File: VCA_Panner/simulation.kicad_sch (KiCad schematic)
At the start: 38 parts, among them U4 TL074, U5 TL074

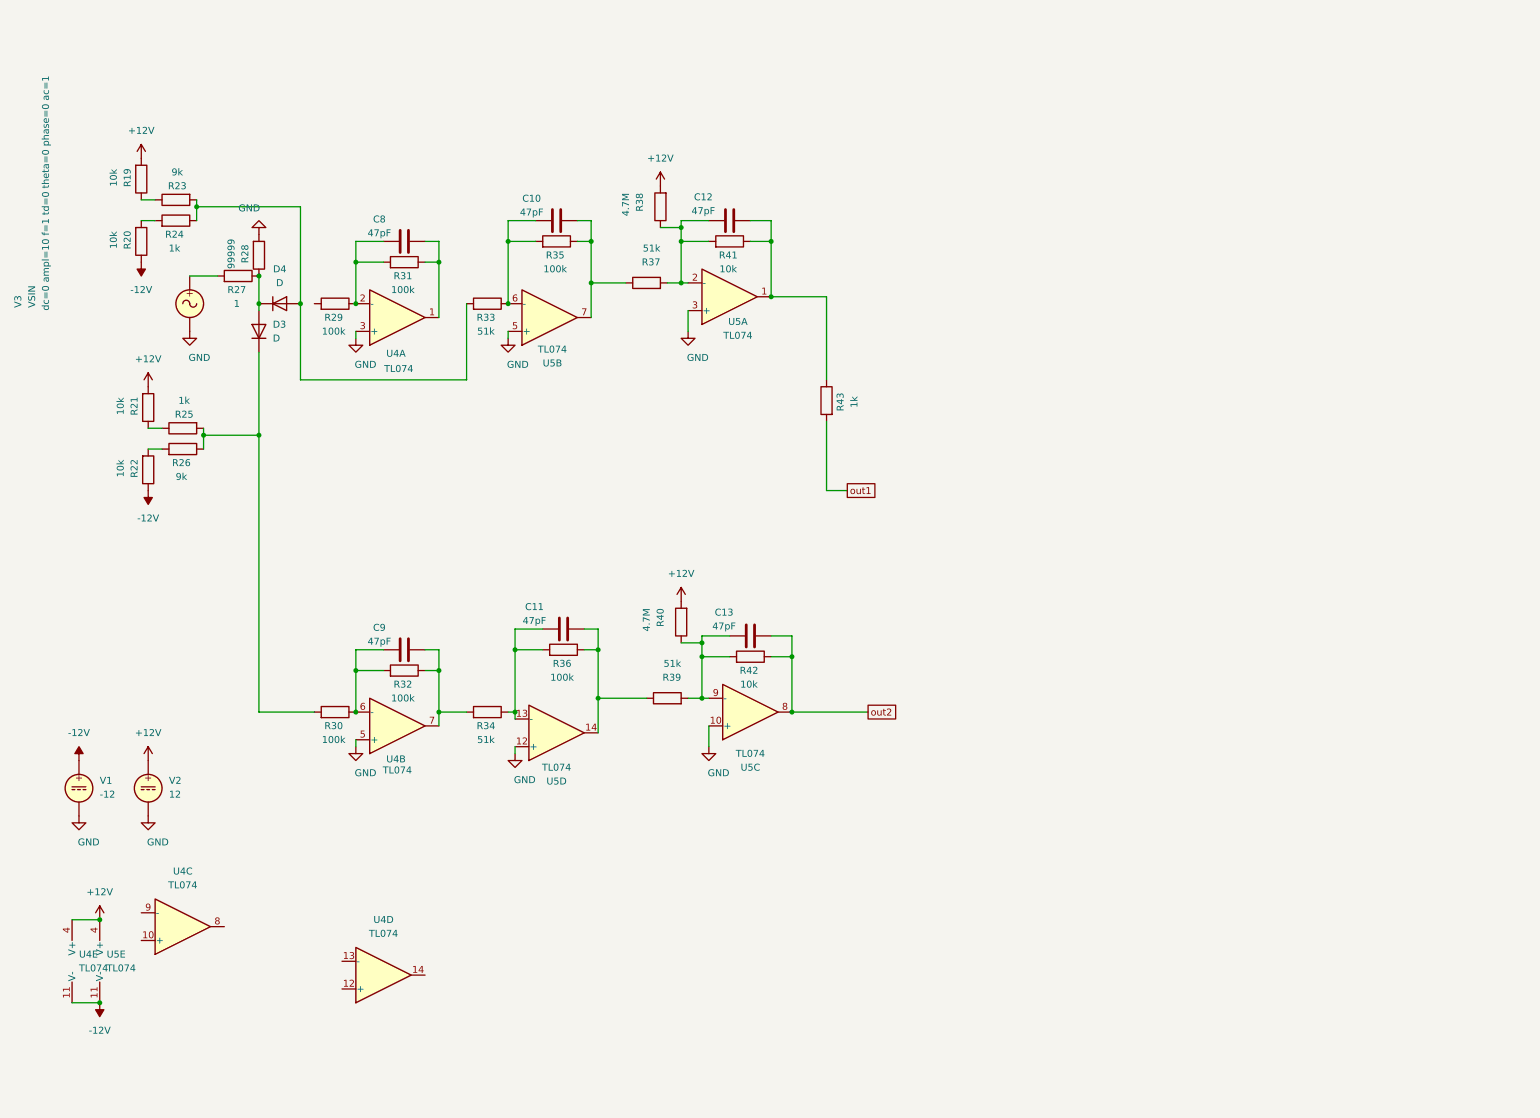
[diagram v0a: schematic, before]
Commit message: feitw bugfixes
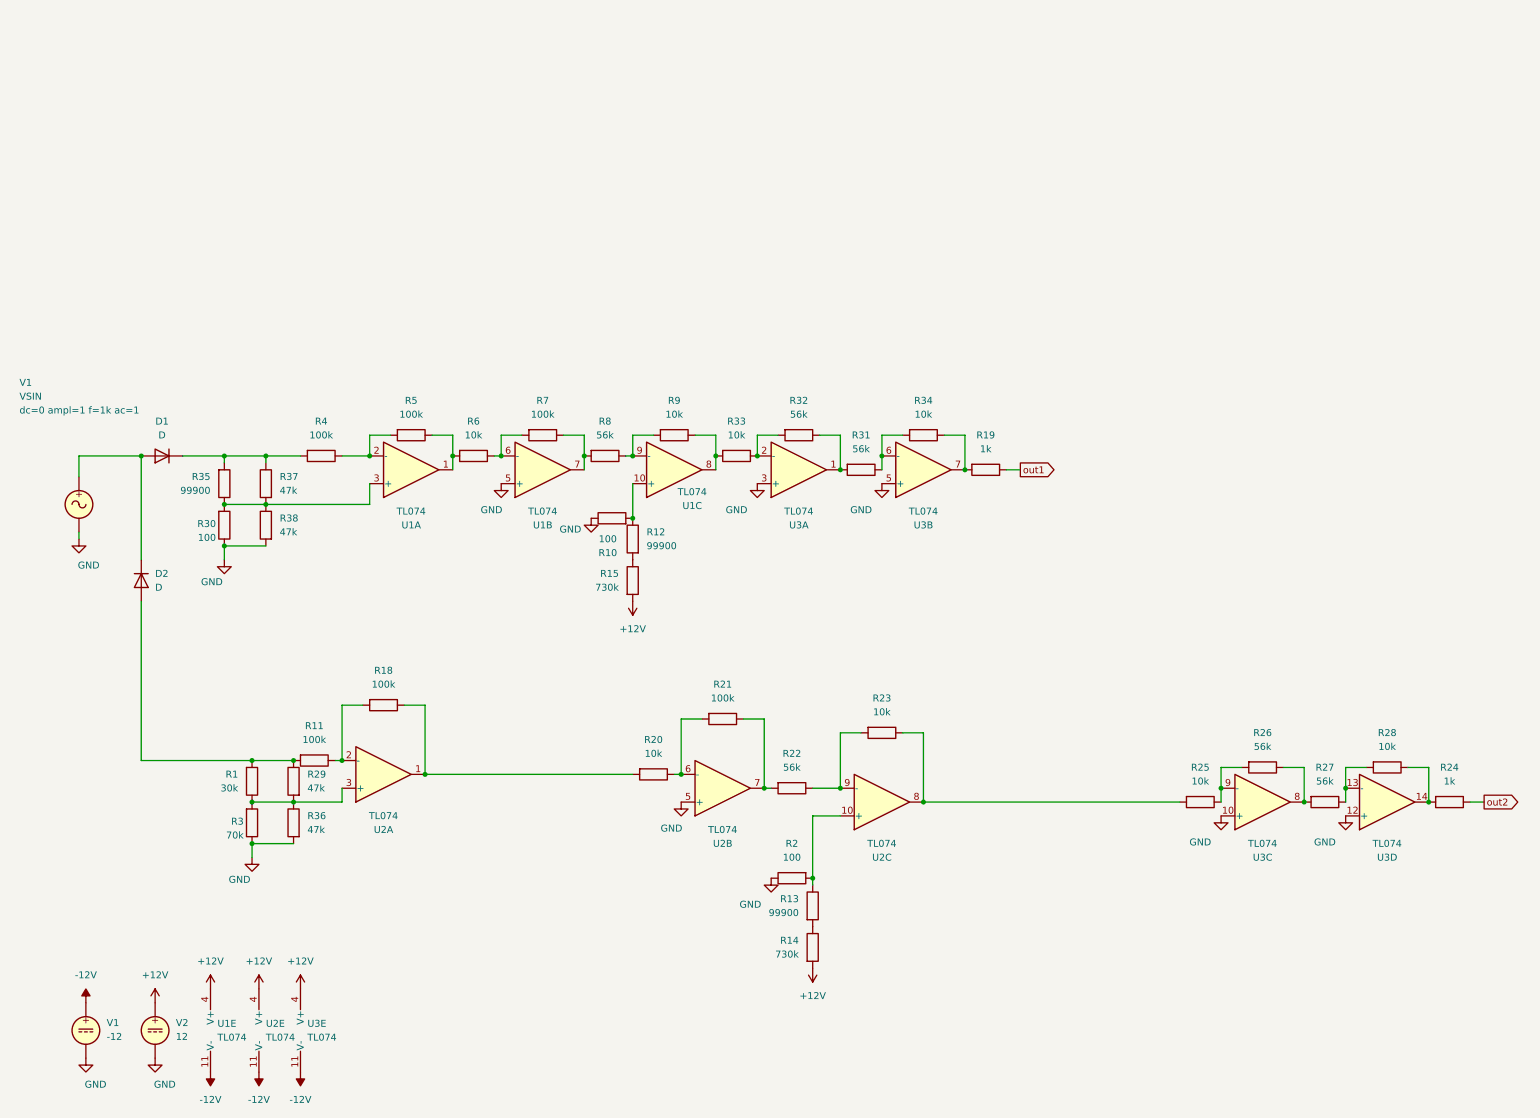
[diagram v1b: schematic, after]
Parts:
- removed C10, C11, C12, C13, C8, C9: 47pF, symbol Device:C
- removed D3, D4: D, symbol Device:D
- removed R39: 51k, symbol Device:R
- removed R40: 4.7M, symbol Device:R
- removed R41, R42: 10k, symbol Device:R
- removed R43: 1k, symbol Device:R
- removed U4, U5: TL074, symbol Amplifier_Operational:TL074
- removed V3: VSIN, symbol Simulation_SPICE:VSIN
- added D1, D2: D, symbol Device:D
- added R1: 30k, symbol Device:R
- added R10, R2: 100, symbol Device:R
- added R11, R18, R4, R5, R7: 100k, symbol Device:R
- added R12, R13: 99900, symbol Device:R
- added R14, R15: 730k, symbol Device:R
- added R3: 70k, symbol Device:R
- added R6, R9: 10k, symbol Device:R
- added R8: 56k, symbol Device:R
- added U1, U2, U3: TL074, symbol Amplifier_Operational:TL074
- added V1: VSIN, symbol Simulation_SPICE:VSIN
- R19: value 10k -> 1k
- R21: value 10k -> 100k
- R22: value 10k -> 56k
- R23: value 9k -> 10k
- R25: value 1k -> 10k
- R26: value 9k -> 56k
- R27: value 1 -> 56k
- R28: value 99999 -> 10k
- R29, R36: value 100k -> 47k
- R30: value 100k -> 100
- R31, R32: value 100k -> 56k
- R33, R34: value 51k -> 10k
- R35: value 100k -> 99900
- R37: value 51k -> 47k
- R38: value 4.7M -> 47k
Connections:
- net +12V: now also R14.2, R15.2, U1.4 (V+), U2.4 (V+), U3.4 (V+); no longer R19.2, R21.2, R38.2
- net -12V: now also U1.11 (V-), U2.11 (V-), U3.11 (V-); no longer R20.1, R22.1
- net GND: now also R30.1, R36.2, R38.2, R10.1, R2.1, R3.1, U1.5 (+), U2.5 (+), U3.10 (+), U3.12 (+), U3.3 (+), U3.5 (+), V1.2; no longer R28.2
- net out1: now also R19.1
- net out2: now also R24.1
- net at R31.1: now also R34.2, U3.6 (-)
- net at R31.2: now also R32.1, U3.1; no longer R29.1
- net at R32.2: now also R33.1, U3.2 (-); no longer R30.1
- net at R23.1: now also R25.2, U2.8; no longer R19.1
- net at R20.2: now also R18.1, U2.1; no longer R24.2
- net at R25.1: now also R26.2, U3.9 (-); no longer R21.1
- net at R27.2: now also R26.1, U3.8
- net at R29.2: now also R36.1, R1.1, R3.2, U2.3 (+)
- net at R37.1: now also R35.2, D1.1 (K), R4.2; no longer R35.1
- net at R37.2, R38.1: now also R30.2, R35.1, U1.3 (+)
- net at R34.1: now also R19.2, U3.7; no longer R36.2
- net at R22.2: now also R21.1, U2.7; no longer R26.2
- net at R27.1: now also R28.2, U3.13 (-); no longer R28.1
- new net: R5.1, R6.2, U1.1
- new net: R4.1, R5.2, U1.2 (-)
- new net: R20.1, R21.2, U2.6 (-)
- new net: R7.1, R8.2, U1.7
- new net: R6.1, R7.2, U1.6 (-)
- new net: R10.2, R12.1, U1.10 (+)
- new net: R12.2, R15.1
- new net: R13.1, R2.2, U2.10 (+)
- new net: R13.2, R14.1
- new net: R24.2, R28.1, U3.14
- new net: R22.1, R23.2, U2.9 (-)
- new net: D1.2 (A), D2.1 (K), V1.1
- new net: D2.2 (A), R1.2, R11.2, R29.1
- new net: R33.2, R9.1, U1.8
- new net: R8.1, R9.2, U1.9 (-)
- new net: R11.1, R18.2, U2.2 (-)
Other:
- moved on the sheet: V1, V2
